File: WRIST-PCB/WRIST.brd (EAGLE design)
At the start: 53 x 17.8 mm, 44 parts, among them Q3 BSS138, U3 LP5907-2.8V

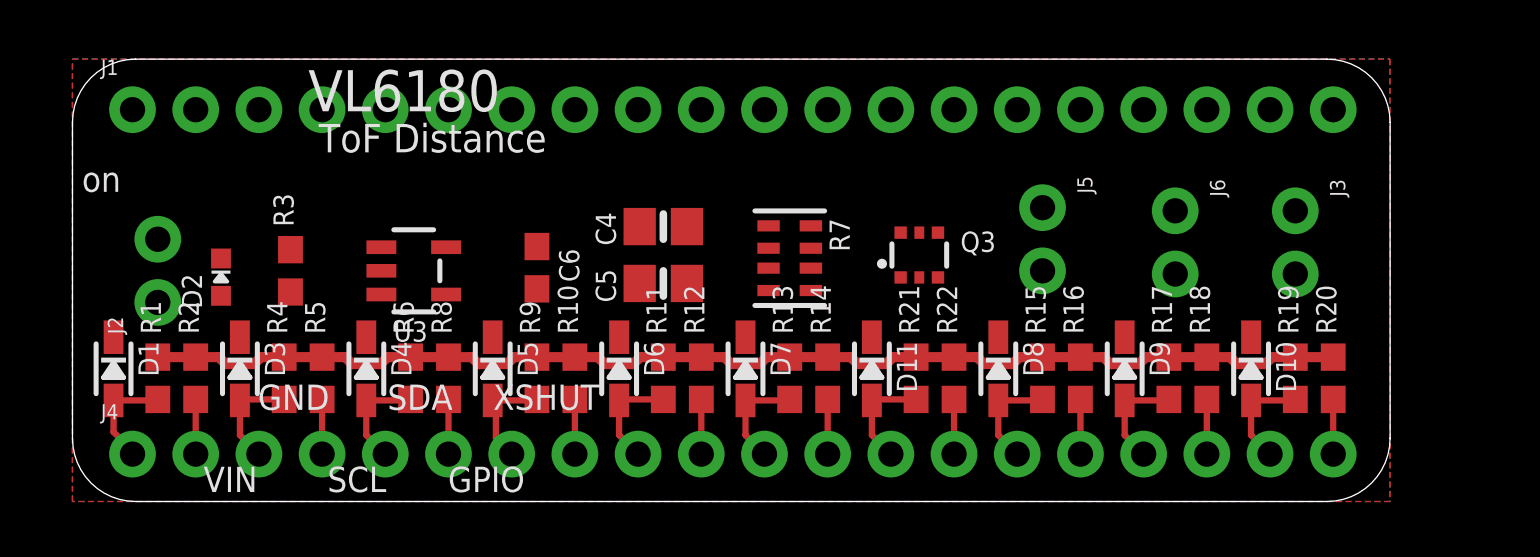
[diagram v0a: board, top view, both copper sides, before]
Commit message: finish wrist pcb
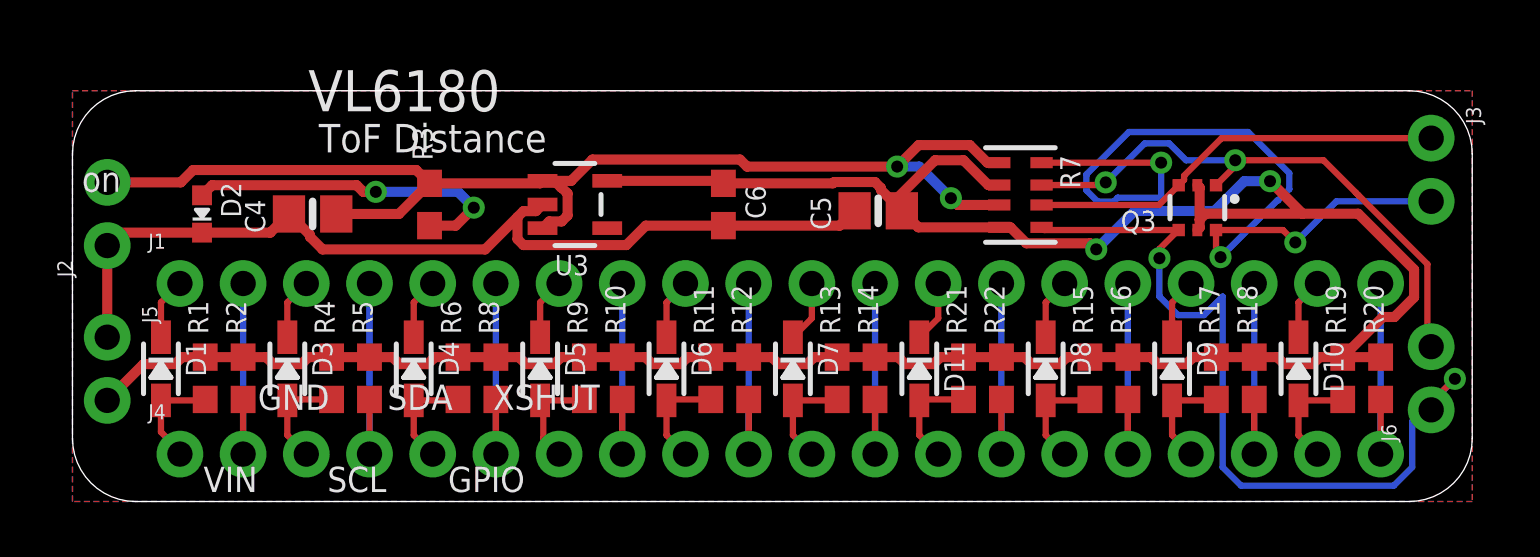
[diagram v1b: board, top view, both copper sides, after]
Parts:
- moved J5 38.0 mm to (1.40, 6.60)
- moved C4 14.1 mm to (9.65, 11.6)
- moved J6 13.0 mm to (54.6, 3.68), turned to 90 degrees
- moved Q3 11.3 mm to (45.2, 11.8), turned to 180 degrees
- moved R7 9.61 mm to (38.1, 12.3)
- moved C5 9.12 mm to (32.4, 11.7)
- moved C6 7.91 mm to (26.2, 11.9)
- moved J1 7.24 mm to (4.32, 8.76)
- moved U3 7.00 mm to (20.2, 11.9)
- moved J3 6.19 mm to (54.6, 14.6)
- moved R3 6.19 mm to (14.4, 11.9)
- moved J2 3.06 mm to (1.40, 10.3)
- moved D2 2.65 mm to (5.21, 11.6), turned to 180 degrees
- moved D10 1.91 mm to (49.3, 5.33)
- moved D11 1.91 mm to (34.0, 5.33)
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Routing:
- net 2.8V: track 49.3 -> 106.7 mm, vias 0 -> 2
- net VCC: track 0.00 -> 49.8 mm, vias 0 -> 2
- net GND: track 0.00 -> 38.2 mm
- net SCL: track 0.00 -> 34.9 mm, vias 0 -> 3
- net SDA_3V: track 0.00 -> 32.7 mm, vias 0 -> 2
- net SCL_3V: track 0.00 -> 22.9 mm, vias 0 -> 2
- net SDA: track 0.00 -> 16.9 mm
- net N$1: track 0.00 -> 13.5 mm, vias 0 -> 2
- net GPIO_9: track 2.20 -> 9.06 mm
- net GPIO_8: track 2.20 -> 9.06 mm
- net GPIO_7: track 2.20 -> 9.06 mm
- net GPIO_6: track 2.20 -> 9.06 mm
- net GPIO_5: track 2.20 -> 9.06 mm
- net GPIO_4: track 2.20 -> 9.06 mm
- net GPIO_3: track 2.20 -> 9.06 mm
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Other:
- board size 53 x 17.8 mm -> 56.3 x 16.5 mm
